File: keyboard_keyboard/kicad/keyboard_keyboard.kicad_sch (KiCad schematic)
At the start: 453 parts, among them J1 AudioJack3_Ground, J2 AudioJack3_Ground, J3 Screen Connector, U1 74HC138

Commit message: routes
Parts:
- U1: footprint (none) -> Package_SO:SOIC-16_3.9x9.9mm_P1.27mm
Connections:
- net +3.3VA: now also R1.2, R2.2, R3.2, U1.16 (VCC)
- net ENB_A: now also A1.5 (SD_DATA_0); no longer A1.4 (SD_DATA_1)
- net ENB_B: now also A1.4 (SD_DATA_1); no longer A1.3 (SD_DATA_2)
- net ENB_C: now also A1.3 (SD_DATA_2); no longer A1.2 (SD_DATA_3)
- net GND: now also U1.7 (~{Y7}), U1.9 (~{Y6})
- net led_2: now reaches D2.1 (K)
- net led_2: now also A1.6 (SD_CMD)
- net led_3: now reaches D3.1 (K)
- net led_3: now also A1.2 (SD_DATA_3)
- net led_1: now reaches D1.1 (K)
- net led_1: now also A1.7 (SD_CLK)
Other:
- moved on the sheet: A1, AM1, AM10, AM11, AM12, AM13, AM14, AM15, AM2, AM3, AM4, AM5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

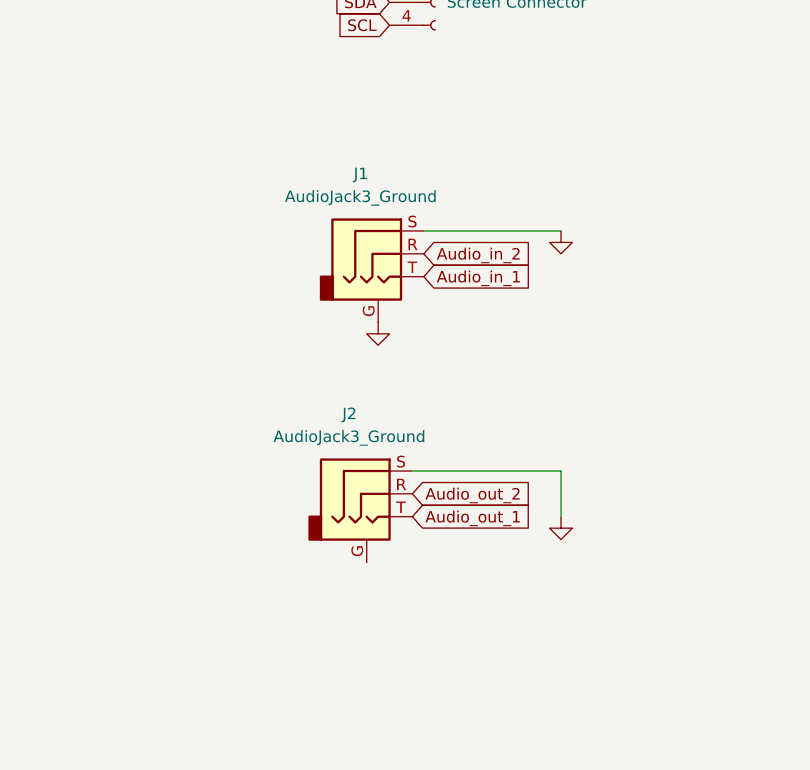
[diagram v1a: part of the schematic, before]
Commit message: more routes
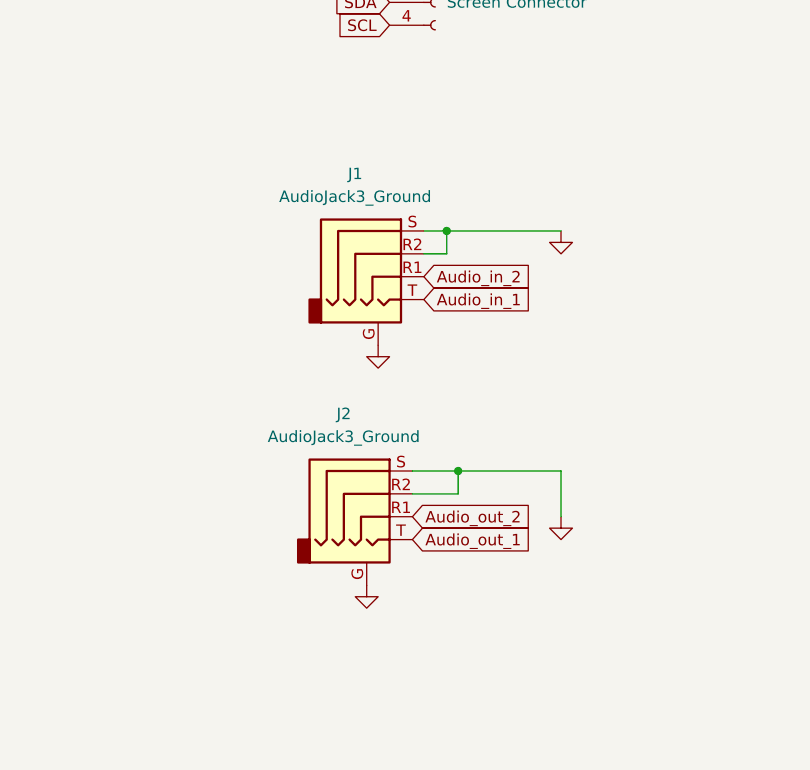
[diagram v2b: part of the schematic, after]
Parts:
- J1, J2: symbol Connector_Audio:AudioJack3_Ground -> Connector_Audio:AudioJack4_Ground
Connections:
- net Audio_in_2: now also J1.R1; no longer J1.R
- net Audio_out_2: now also J2.R1; no longer J2.R
- net GND: now also J1.R2, J2.G, J2.R2

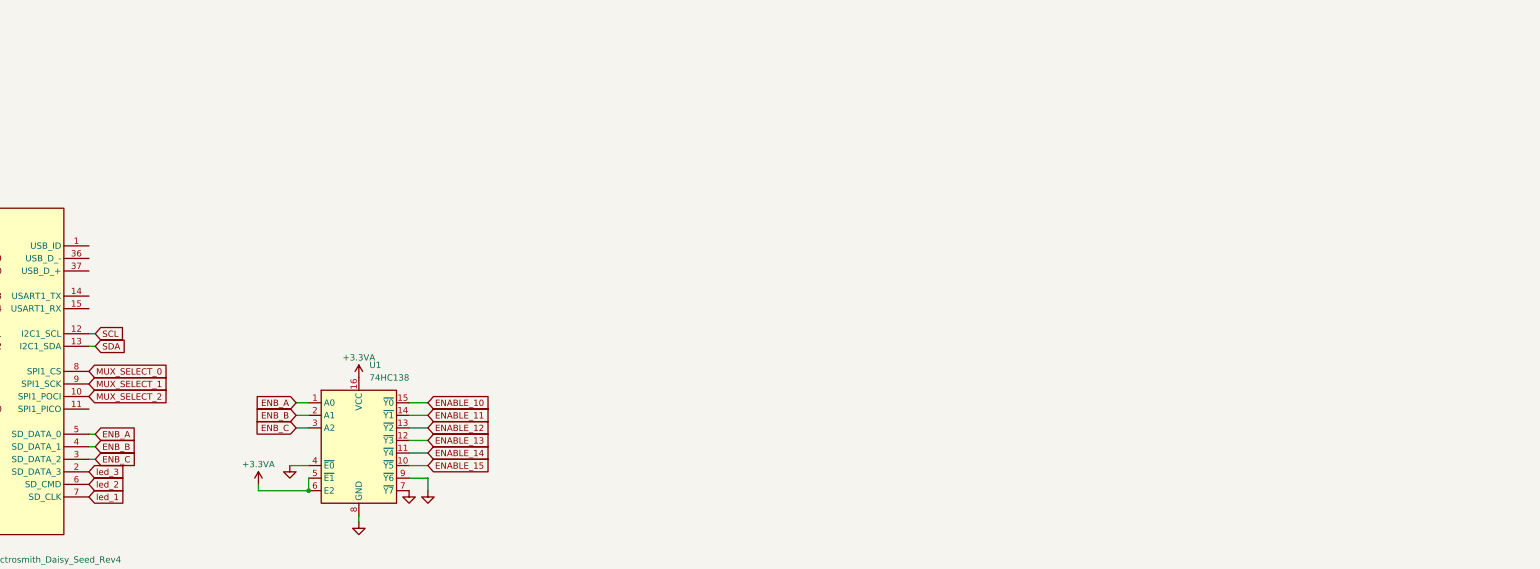
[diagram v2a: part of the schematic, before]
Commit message: add routes
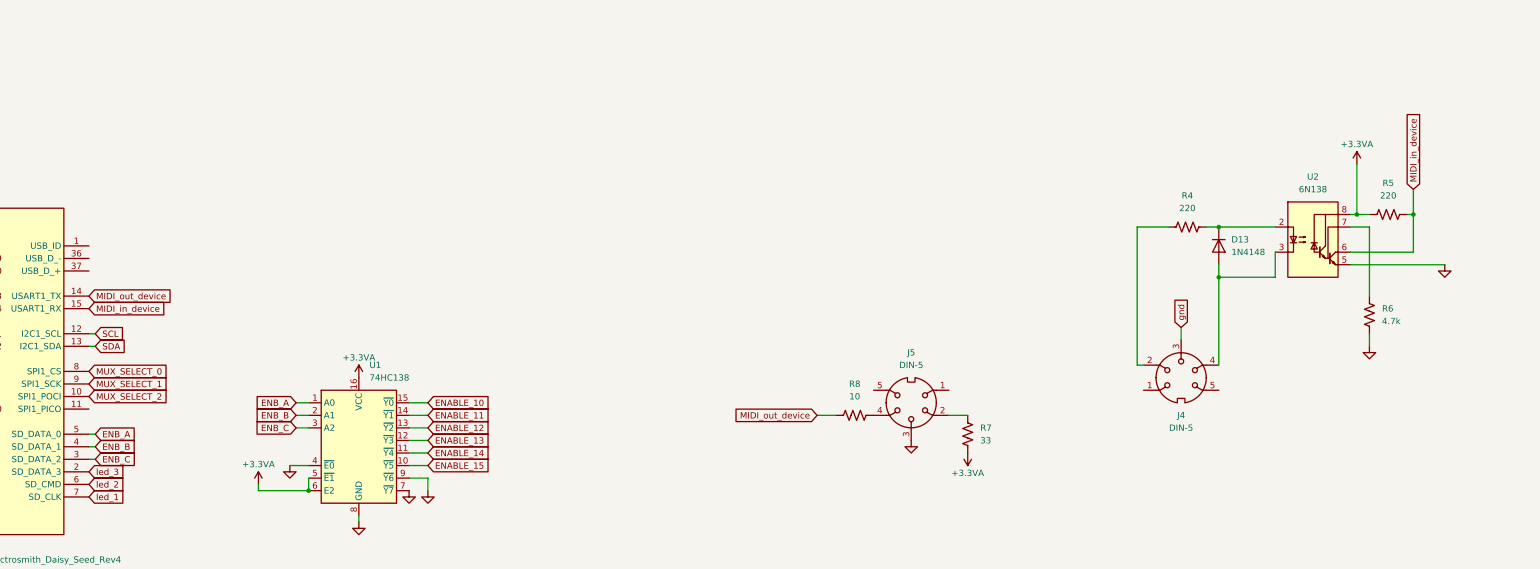
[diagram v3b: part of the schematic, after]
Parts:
- added D13: 1N4148, Diode_THT:D_DO-35_SOD27_P7.62mm_Horizontal, symbol Diode:1N4148
- added J4, J5: DIN-5, Connector_JST:JST_PH_B5B-PH-K_1x05_P2.00mm_Vertical, symbol Connector:DIN-5
- added R4, R5: 220, Resistor_THT:R_Axial_DIN0207_L6.3mm_D2.5mm_P15.24mm_Horizontal, symbol Device:R_US
- added R6: 4.7k, Resistor_THT:R_Axial_DIN0207_L6.3mm_D2.5mm_P15.24mm_Horizontal, symbol Device:R_US
- added R7: 33, Resistor_THT:R_Axial_DIN0207_L6.3mm_D2.5mm_P15.24mm_Horizontal, symbol Device:R_US
- added R8: 10, Resistor_THT:R_Axial_DIN0207_L6.3mm_D2.5mm_P15.24mm_Horizontal, symbol Device:R_US
- added U2: 6N138, Package_DIP:DIP-8_W7.62mm, symbol Isolator:6N138
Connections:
- net +3.3VA: now also R5.2, R7.1, U2.8 (VCC)
- net GND: now also J5.3, R6.1, U2.5 (GND)
- net MIDI_out_device: now reaches A1.14 (USART1_TX)
- net MIDI_out_device: now also R8.1
- net MIDI_in_device: now reaches A1.15 (USART1_RX)
- net MIDI_in_device: now also R5.1, U2.6 (VO2)
- new net: J4.2, R4.1
- new net: D13.1 (K), R4.2, U2.2 (C1)
- new net: J5.2, R7.2
- new net: R6.2, U2.7 (VO1)
- new net: J5.4, R8.2
- new net: D13.2 (A), J4.4, U2.3 (C2)
- new net gnd: J4.3
